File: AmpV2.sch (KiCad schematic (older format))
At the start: 1 part

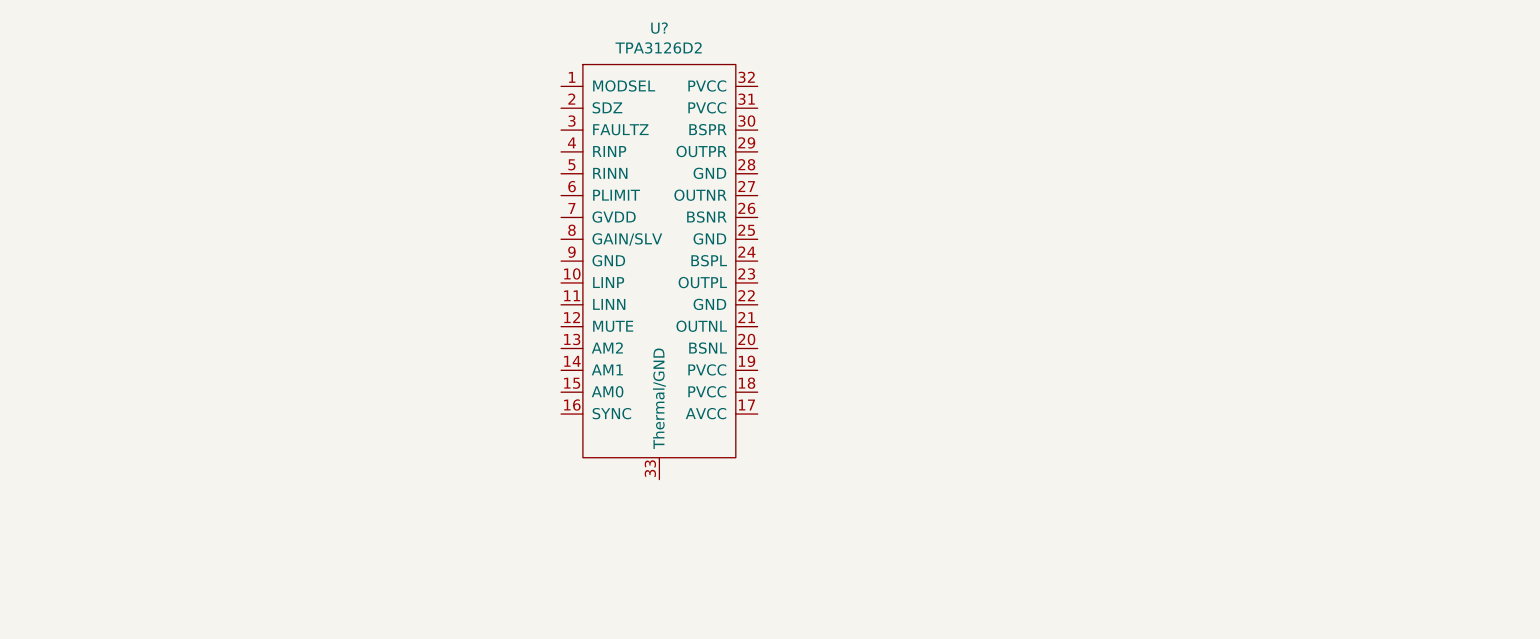
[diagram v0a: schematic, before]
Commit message: making layout
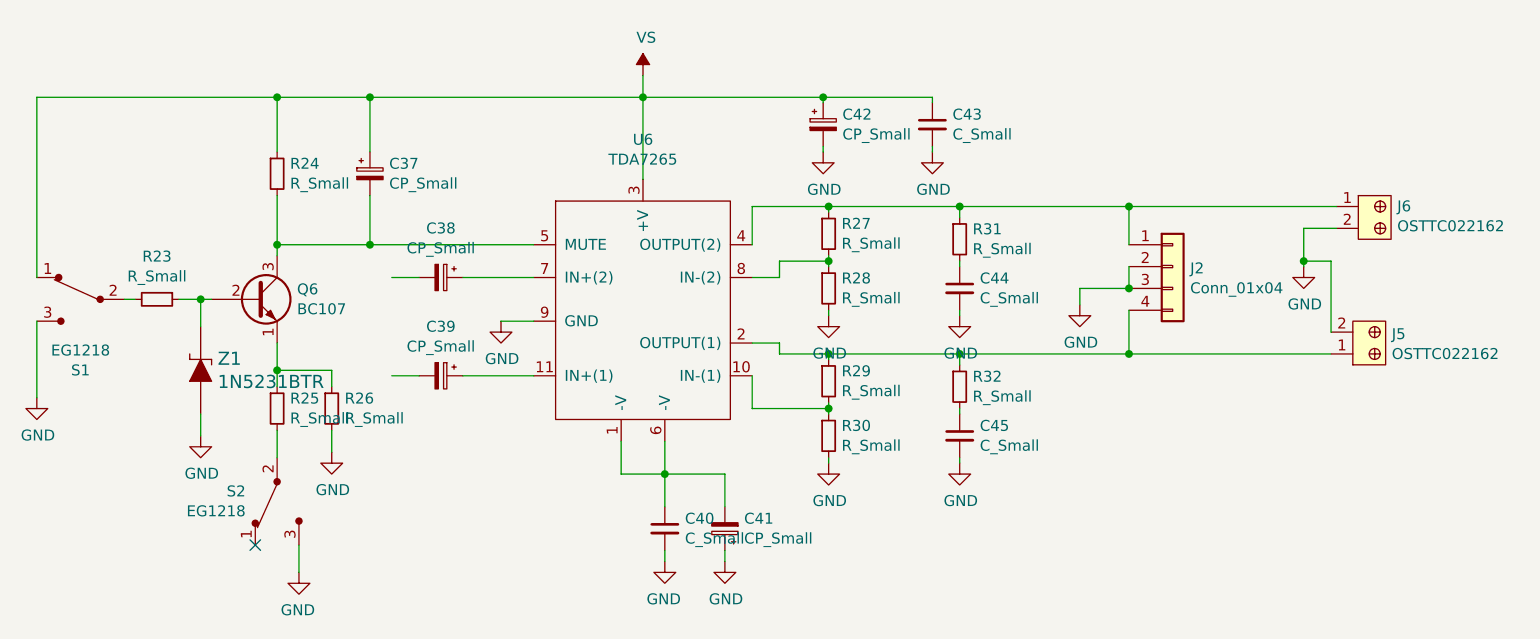
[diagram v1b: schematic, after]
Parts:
- removed U?: TPA3126D2, Package_SO:HTSSOP-32-1EP_6.1x11mm_P0.65mm_EP5.2x11mm_Mask4.11x4.36mm, symbol CustomLibrary:TPA3126D2
- added C37, C38, C39, C41, C42: CP_Small, Capacitor_SMD:C_0603_1608Metric_Pad1.08x0.95mm_HandSolder, symbol Device:CP_Small
- added C40, C43, C44, C45: C_Small, Capacitor_SMD:C_0603_1608Metric_Pad1.08x0.95mm_HandSolder, symbol Device:C_Small
- added J2: Conn_01x04, Connector_JST:JST_PH_S4B-PH-K_1x04_P2.00mm_Horizontal, symbol Connector_Generic:Conn_01x04
- added J5, J6: OSTTC022162, digikey-footprints:Term_Block_1x2_P5.08MM, symbol dk_Terminal-Blocks-Wire-to-Board:OSTTC022162
- added Q6: BC107, Package_TO_SOT_THT:TO-18-3, symbol Transistor_BJT:BC107
- added R23, R24, R25, R26, R27, R28, R29, R30, R31, R32: R_Small, Resistor_SMD:R_0603_1608Metric_Pad0.98x0.95mm_HandSolder, symbol Device:R_Small
- added S1, S2: EG1218, digikey-footprints:Switch_Slide_11.6x4mm_EG1218, symbol dk_Slide-Switches:EG1218
- added U6: TDA7265, Package_TO_SOT_THT:TO-220-11_P3.4x5.08mm_StaggerOdd_Lead4.85mm_Vertical, symbol CustomLibrary:TDA7265
- added Z1: 1N5231BTR, digikey-footprints:DO-35, symbol dk_Diodes-Zener-Single:1N5231BTR
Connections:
- new net: C40.1, C41.2, U6.1 (-V), U6.6 (-V)
- new net: R29.2, R30.1, U6.10 (IN-(1))
- new net: C39.1, U6.11 (IN+(1))
- new net: J2.4 (Pin_4), J5.1, R29.1, R32.1, U6.2 (OUTPUT(1))
- new net: J2.1 (Pin_1), J6.1, R27.1, R31.1, U6.4 (OUTPUT(2))
- new net: C37.2, Q6.3 (C), R24.2, U6.5 (MUTE)
- new net: C38.1, U6.7 (IN+(2))
- new net: R27.2, R28.1, U6.8 (IN-(2))
- new net: Q6.1 (E), R25.1, R26.1
- new net: Q6.2 (B), R23.1, Z1.K
- new net: R25.2, S2.2
- new net: R23.2, S1.2
- new net: C44.1, R31.2
- new net: C45.1, R32.2
- new net GND: C40.2, C41.1, C42.2, C43.2, C44.2, C45.2, J2.2 (Pin_2), J2.3 (Pin_3), J5.2, J6.2, R26.2, R28.2, R30.2, S1.3, S2.3, U6.9 (GND), Z1.A
- new net VS: C37.1, C42.1, C43.1, R24.1, S1.1, U6.3 (+V)
- no-connect marks 0 -> 1
